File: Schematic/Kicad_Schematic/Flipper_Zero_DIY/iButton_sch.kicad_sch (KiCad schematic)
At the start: 1 part, among them J1 Conn_01x06_Socket

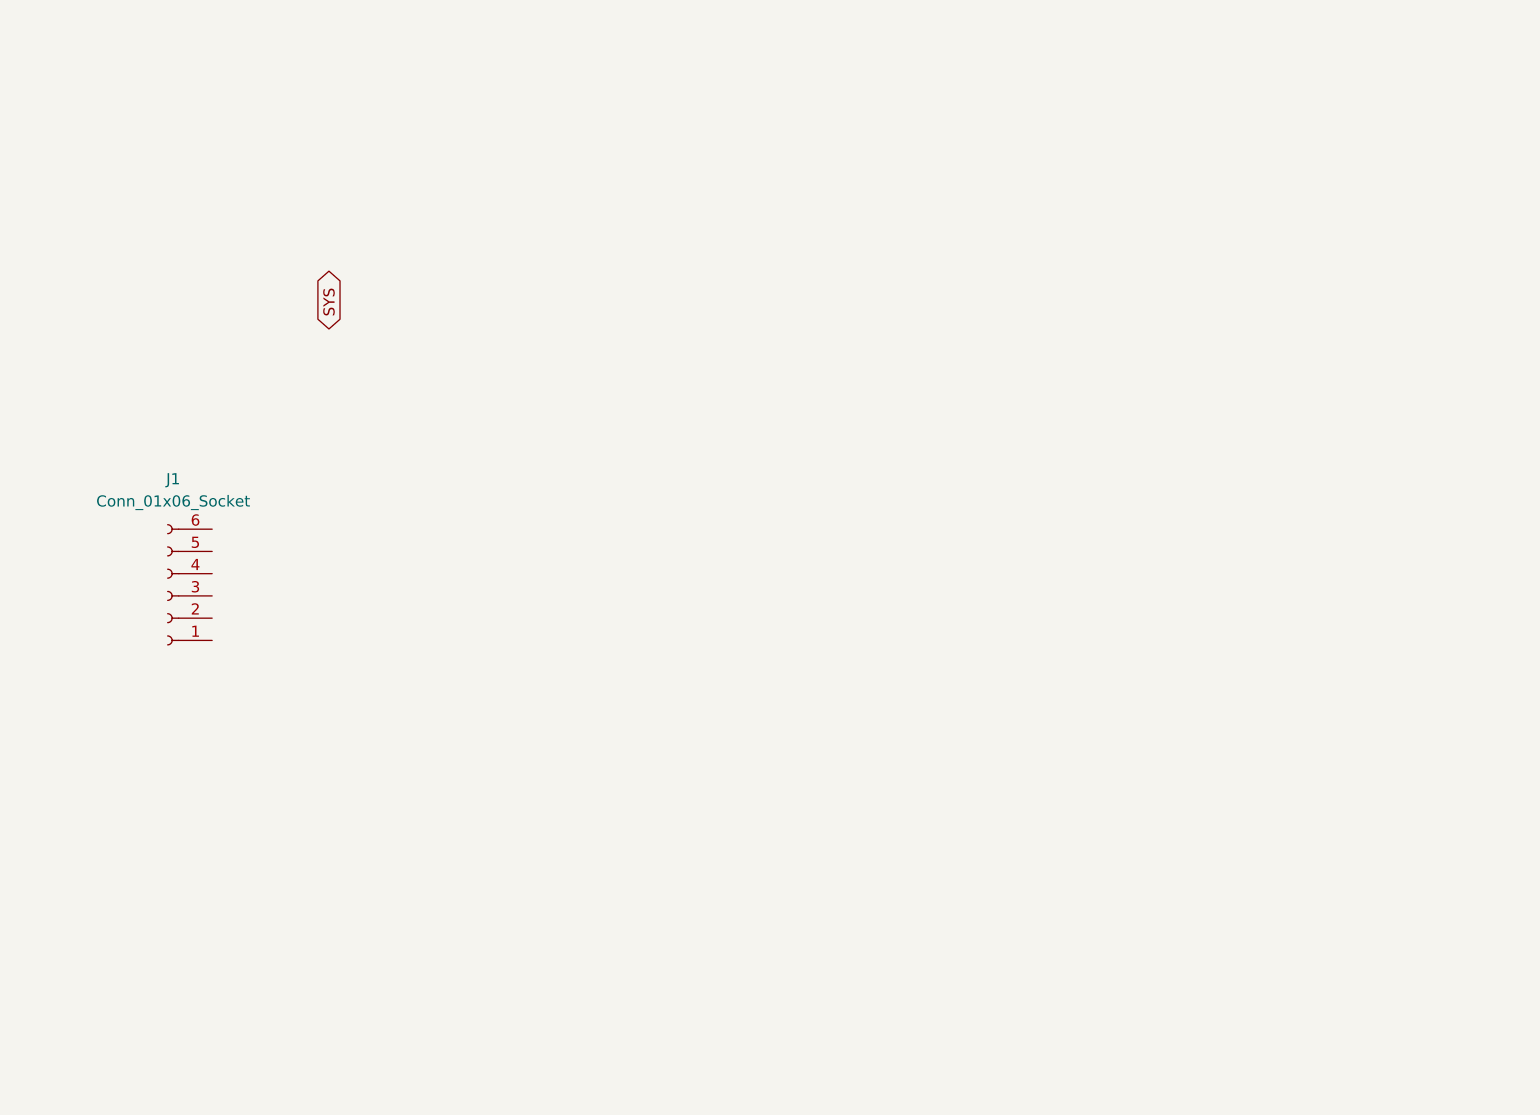
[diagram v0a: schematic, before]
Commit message: finished iBtn PCB
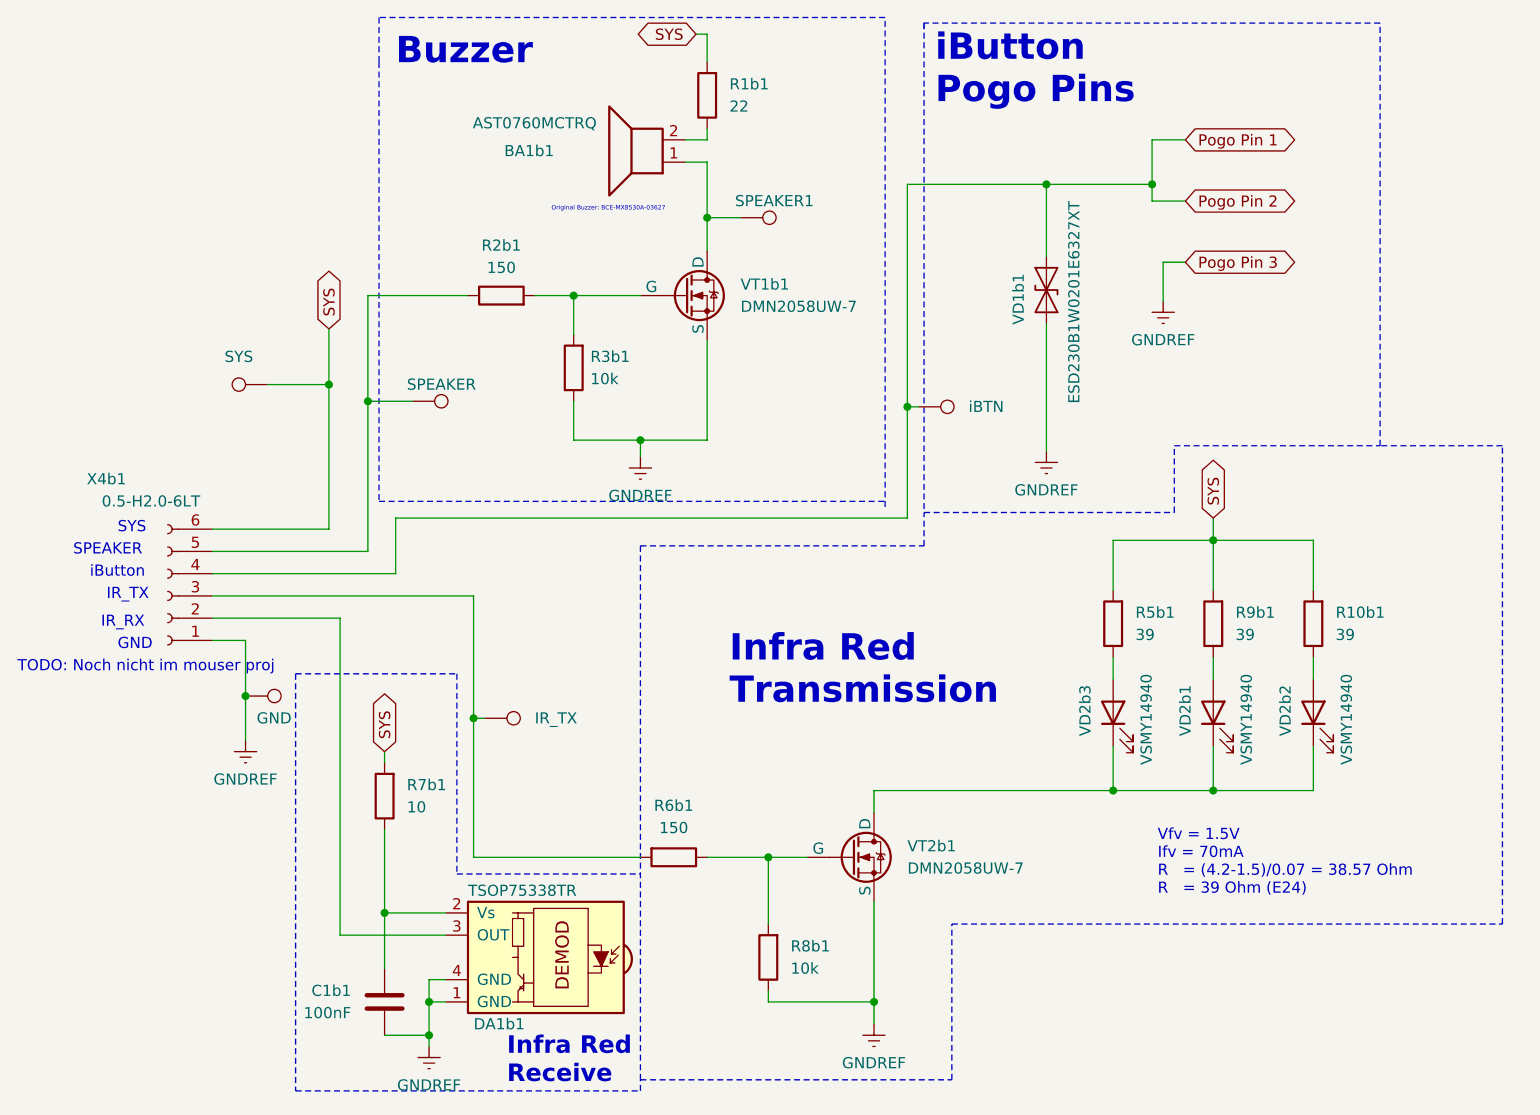
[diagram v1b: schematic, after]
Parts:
- added BA1b1: AST0760MCTRQ, footprints:Buzzer_539-AST0760MCTRQ, symbol Device:Speaker
- added C1b1: 100nF, Capacitor_SMD:C_0402_1005Metric, symbol Device:C
- added DA1b1: TSOP75338TR, footprints:TSOP75338TR, symbol Interface_Optical:TSOP21xx
- added R10b1, R5b1, R9b1: 39, Resistor_SMD:R_0402_1005Metric, symbol Device:R
- added R1b1: 22, Resistor_SMD:R_0603_1608Metric, symbol Device:R
- added R2b1, R6b1: 150, Resistor_SMD:R_0402_1005Metric, symbol Device:R
- added R3b1, R8b1: 10k, Resistor_SMD:R_0402_1005Metric, symbol Device:R
- added R7b1: 10, Resistor_SMD:R_0402_1005Metric, symbol Device:R
- added TP56: SYS, TestPoint:TestPoint_Pad_1.0x1.0mm, symbol Connector:TestPoint
- added TP57: SPEAKER, TestPoint:TestPoint_Pad_1.0x1.0mm, symbol Connector:TestPoint
- added TP58: SPEAKER1, TestPoint:TestPoint_Pad_1.0x1.0mm, symbol Connector:TestPoint
- added TP59: iBTN, TestPoint:TestPoint_Pad_1.0x1.0mm, symbol Connector:TestPoint
- added TP60: IR_TX, TestPoint:TestPoint_Pad_1.0x1.0mm, symbol Connector:TestPoint
- added TP61: GND, TestPoint:TestPoint_Pad_1.0x1.0mm, symbol Connector:TestPoint
- added VD1b1: ESD230B1W0201E6327XT, Diode_SMD:D_SOD-923, symbol Diode:ESD9B3.3ST5G
- added VD2b1, VD2b2, VD2b3: VSMY14940, LED_SMD:LED_0603_1608Metric, symbol Device:LED
- added VT1b1, VT2b1: DMN2058UW-7, footprints:SOT323_DMN2058UW_DIO, symbol Simulation_SPICE:NMOS
- X4b1: renamed from J1; value Conn_01x06_Socket -> 0.5-H2.0-6LT; footprint (none) -> Connector_JST:JST_SH_SM06B-SRSS-TB_1x06-1MP_P1.00mm_Horizontal
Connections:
- net SYS: now also X4b1.6 (Pin_6), R10b1.2, R1b1.2, R5b1.2, R7b1.2, R9b1.2, TP56.1
- net GNDREF: now reaches X4b1.1 (Pin_1)
- net GNDREF: now also C1b1.2, DA1b1.1 (GND), DA1b1.4 (GND), R3b1.1, R8b1.1, TP61.1, VD1b1.1 (A1), VT1b1.3 (S), VT2b1.3 (S)
- net at X4b1.2 (Pin_2): now also DA1b1.3 (OUT)
- net at X4b1.3 (Pin_3): now also R6b1.2, TP60.1
- net Pogo Pin 1: now reaches X4b1.4 (Pin_4)
- net Pogo Pin 1: now also TP59.1, VD1b1.2 (A2)
- net at X4b1.5 (Pin_5): now also R2b1.1, TP57.1
- new net: R6b1.1, R8b1.2, VT2b1.2 (G)
- new net: VD2b1.1 (K), VD2b2.1 (K), VD2b3.1 (K), VT2b1.1 (D)
- new net: R10b1.1, VD2b2.2 (A)
- new net: BA1b1.1, TP58.1, VT1b1.1 (D)
- new net: R2b1.2, R3b1.2, VT1b1.2 (G)
- new net: C1b1.1, DA1b1.2 (Vs), R7b1.1
- new net: R9b1.1, VD2b1.2 (A)
- new net: R5b1.1, VD2b3.2 (A)
- new net: BA1b1.2, R1b1.1
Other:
- note added: "Buzzer"
- note added: "GND"
- note added: "IR_RX"
- note added: "IR_TX"
- note added: "Infra Red Receive"
- note added: "Infra Red Transmission"
- note added: "Original Buzzer: BCE-MX8530A-03627"
- note added: "SPEAKER"
- note added: "SYS"
- note added: "TODO: Noch nicht im mouser proj"
- note added: "Vfv = 1.5V Ifv = 70mA R = (4.2-1.5)/0.07 = 38.57 Ohm R = 39 Ohm (E24)"
- note added: "iButton"
- note added: "iButton Pogo Pins"
